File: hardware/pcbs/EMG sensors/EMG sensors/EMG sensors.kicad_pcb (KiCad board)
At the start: 4 copper layers, 90.3 x 73 mm, 27 parts, among them IC1 INA128, J1 Conn_01x04_Pin, U6 OPA2188AIDR, U7 OPA188AIDR

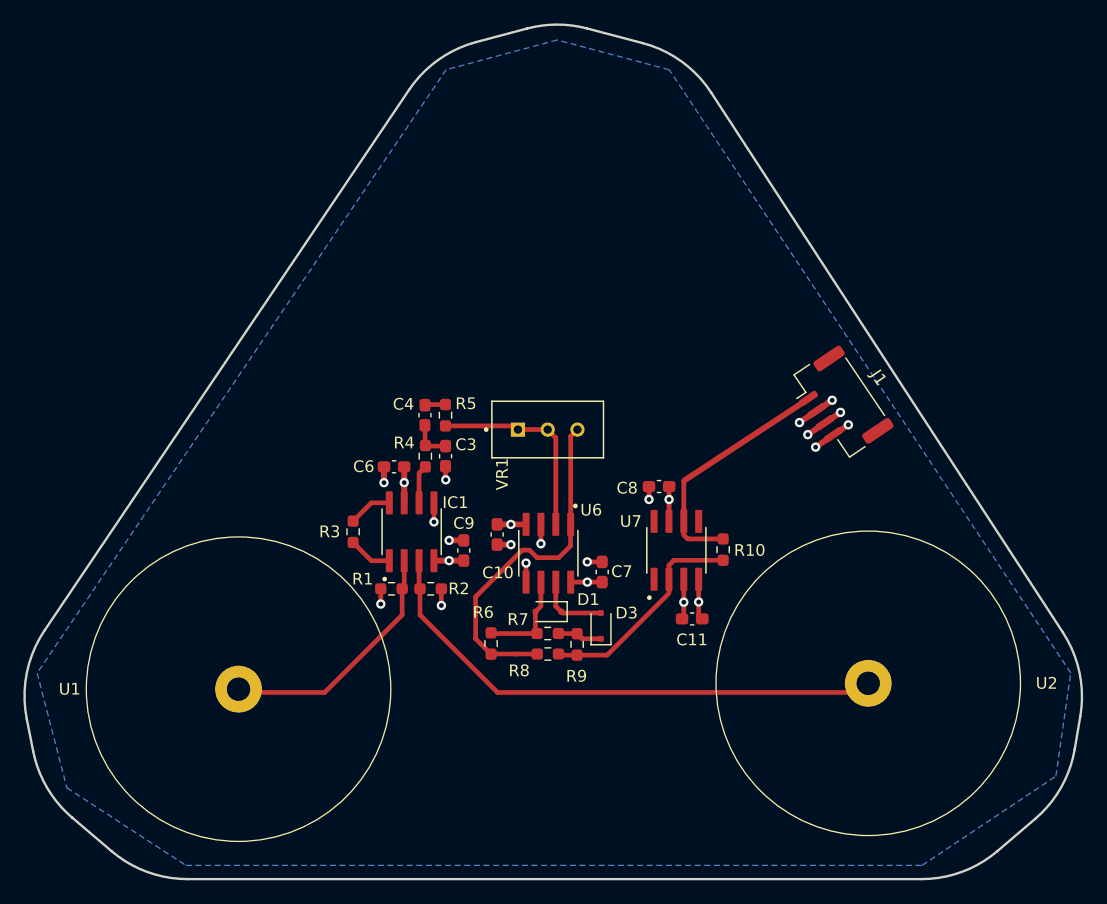
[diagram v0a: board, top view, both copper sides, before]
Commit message: EMG sensor v0.2
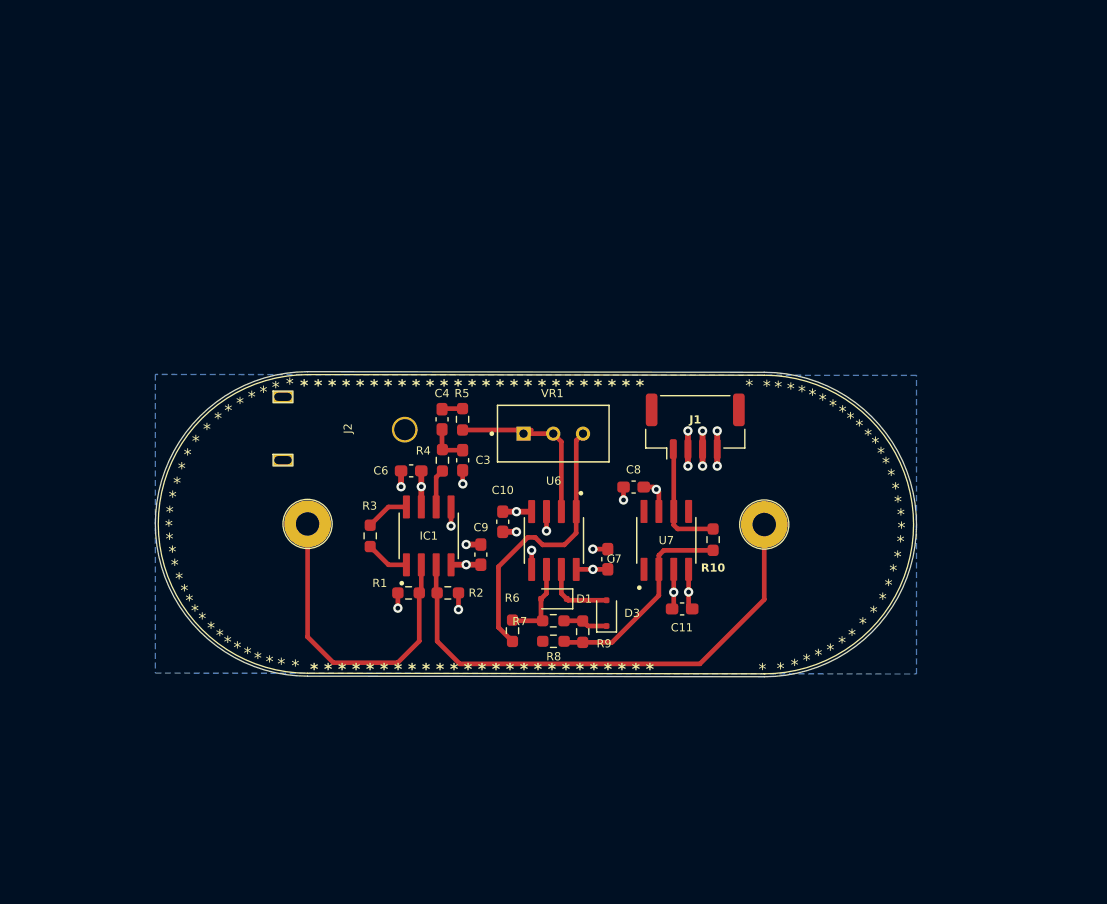
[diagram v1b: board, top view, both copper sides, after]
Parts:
- added J2: Conn_01x01_Pin, Connectors:DIN_Male_1PIN_1.5mm, F.Cu at (110.9, 103.6)
- U1, U2: moved to B.Cu
- moved U2 16.2 mm to (151.0, 110.6)
- moved U1 15.3 mm to (112.0, 110.5)
- moved J1 12.5 mm to (145.1, 102.2), turned to 0 degrees
- moved C8 2.18 mm to (139.8, 107.4)
- moved R6 2.13 mm to (129.5, 119.7)
- moved R5 1.50 mm to (125.2, 101.6)
- moved R2 1.50 mm to (124.0, 116.4)
- moved C9 1.50 mm to (126.8, 113.2)
- moved IC1 1.50 mm to (122.3, 111.6)
- moved R3 1.50 mm to (117.3, 111.6)
- moved C3 1.50 mm to (125.2, 105.1)
- moved C4 1.50 mm to (123.5, 101.6)
- moved C6 1.50 mm to (120.8, 106.0)
- moved R1 1.50 mm to (120.6, 116.4)
- moved R4 1.50 mm to (123.5, 105.1)
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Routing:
- net INVERTED: track 30.0 -> 24.0 mm
- net Vin2: track 46.4 -> 42.0 mm
- net /+5.5V: track 9.04 -> 12.7 mm
- net Ref: track 18.6 -> 21.6 mm
- net /-5.5V: track 8.53 -> 11.5 mm
- net Vin1: track 22.8 -> 25.5 mm
- net Net-(U6--INA): track 17.3 -> 15.9 mm
- net Net-(D1-A): track 8.92 -> 7.57 mm
- net /AEMG: track 9.34 -> 10.2 mm
- net Net-(U7--IN): track 18.9 -> 18.2 mm
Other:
- board size 90.3 x 73 mm -> 65 x 26 mm
- board text added: "*"
- board text added: "* * * * * * * * * * * * * * * * * * * * * * * * *"
